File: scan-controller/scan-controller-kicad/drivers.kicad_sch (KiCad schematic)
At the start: 52 parts, among them CN2 Motor, CN3 Fan, CN4 Lamp, Q1 CS12N06AE-G, U10 LGS5145, U11 MCP1416, U3 78L05, U4 DRV8871DDA, U6 TL431, U7 XL4015, U8 LM358

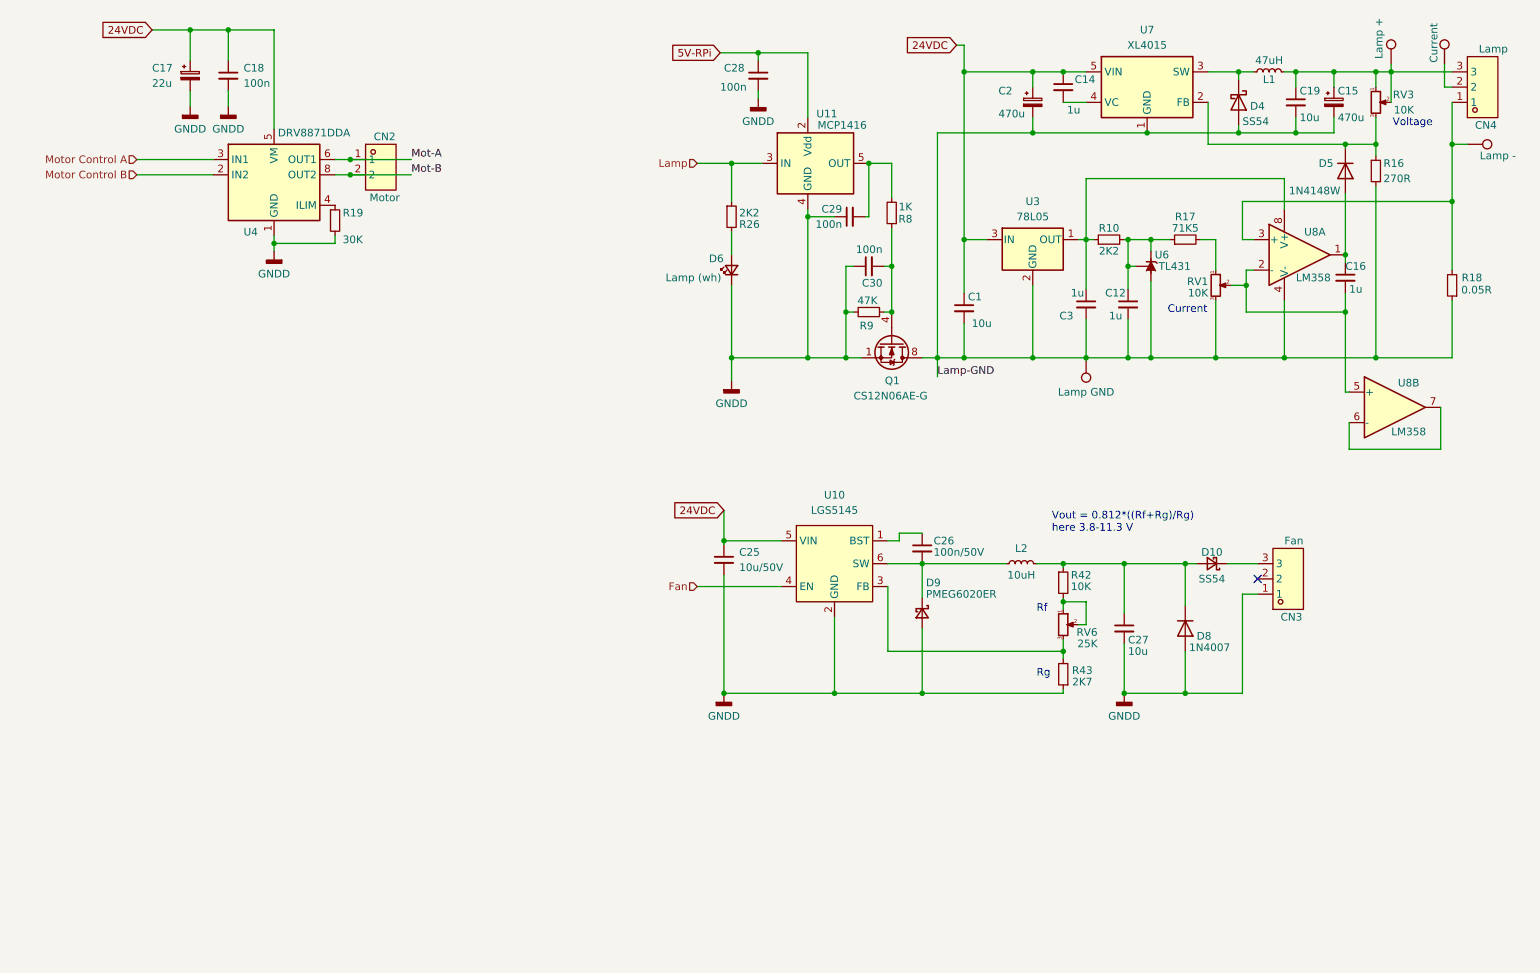
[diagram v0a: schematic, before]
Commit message: Major refactoring to better EMV in progress
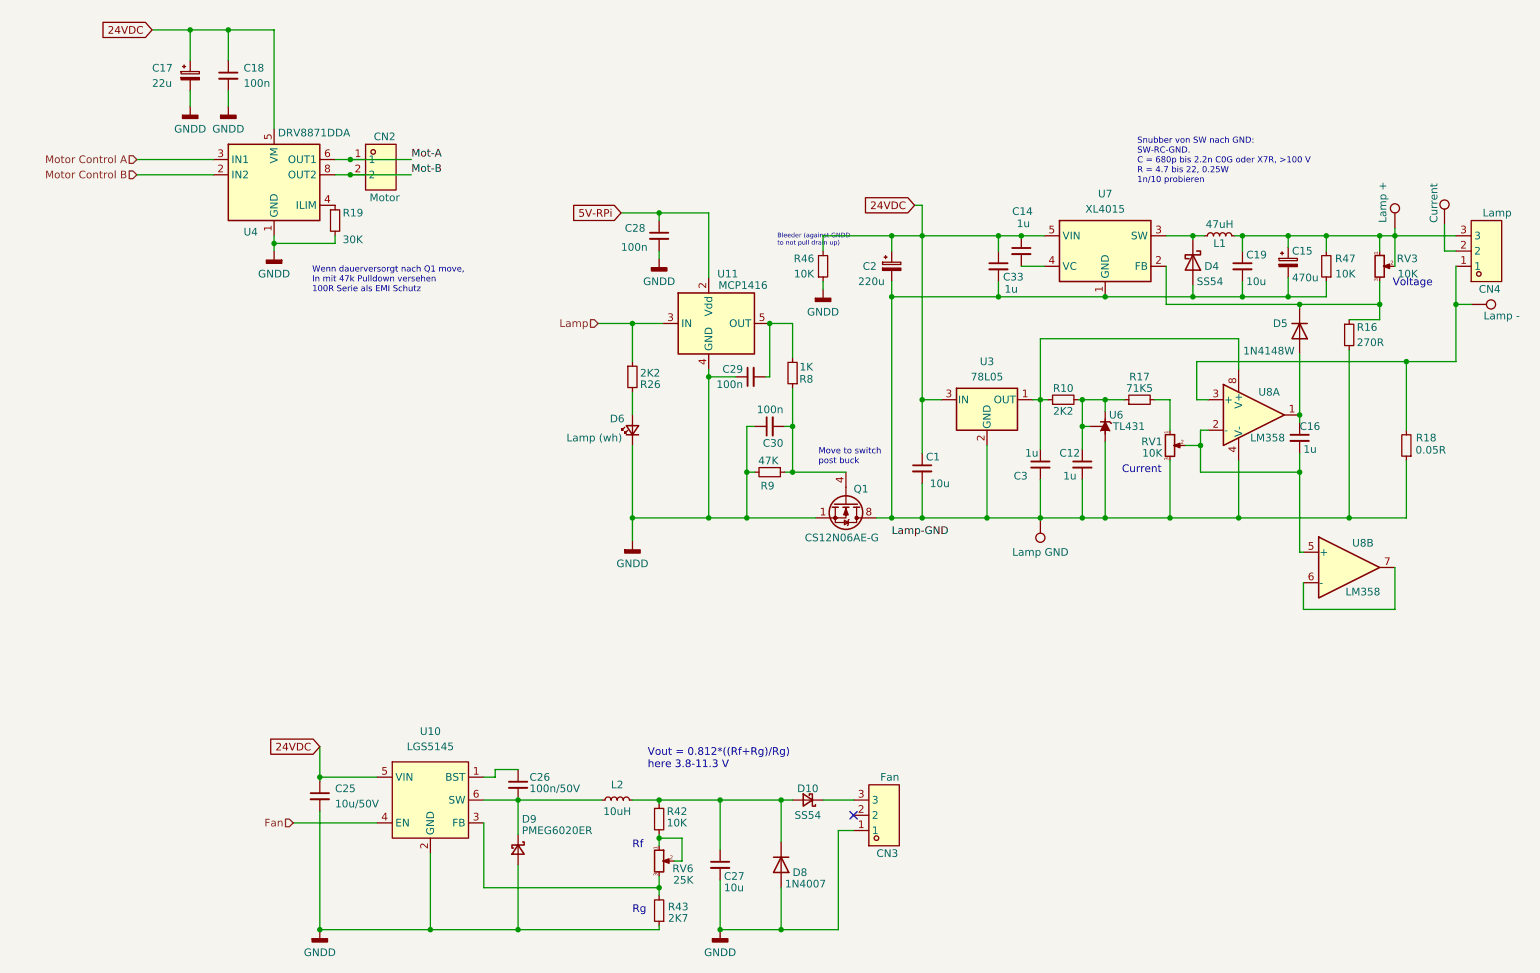
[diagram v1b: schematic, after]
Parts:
- added C33: 1u, Capacitor_SMD:C_0805_2012Metric, symbol Device:C_Small
- added R46, R47: 10K, Resistor_SMD:R_1206_3216Metric, symbol Device:R_Small
- C2: value 470u -> 220u; LCSC C90272 -> (none)
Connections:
- net 24VDC: now also C33.1, R46.2
- net GNDD: now also R46.1
- net Lamp-GND: no longer C1.2, C12.2, C15.2, C19.2, C2.2, C3.2, D4.2 (A), Q1.5 (D), Q1.6 (D), Q1.7 (D), Q1.8 (D), R16.2, R18.1, RV1.3, TP9.1, U3.2 (GND), U6.3 (A), U7.1 (GND), U8.4 (V-)
- net at C15.1, C19.1, CN4.3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: now also R47.2
- new net: C1.2, C12.2, C15.2, C19.2, C2.2, C3.2, C33.2, D4.2 (A), Q1.5 (D), Q1.6 (D), Q1.7 (D), Q1.8 (D), R16.2, R18.1, R47.1, RV1.3, TP9.1, U3.2 (GND), U6.3 (A), U7.1 (GND), U8.4 (V-)
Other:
- note added: "Bleeder (against GNDD to not pull drain up)"
- note added: "Move to switch post buck"
- note added: "Snubber von SW nach GND: SW-RC-GND. C = 680p bis 2.2n C0G oder X7R, >100 V R = 4.7 bis 22, 0.25W 1n/10 probieren"
- note added: "Wenn dauerversorgt nach Q1 move, In mit 47k Pulldown versehen 100R Serie als EMI Schutz"
- moved on the sheet: C1, C12, C14, C15, C16, C19, C2, C25, C26, C27, C28, C29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
